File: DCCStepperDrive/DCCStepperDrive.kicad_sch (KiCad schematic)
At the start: 34 parts, among them J1 12v, J2 CBUS, J3 5V select, J4 DCC, J5 Grove 2mm, J6 GROVE-CONNECTOR-DIP_4P-2.0_, J7 Sensor, J8 Motor, J9 Mode Select, Q1 DMG2305UX-7, SW1 SW_Push, U1 AMS1117-3.3, U2 AMS1117-5.0, U3 6N137, U4 Pico

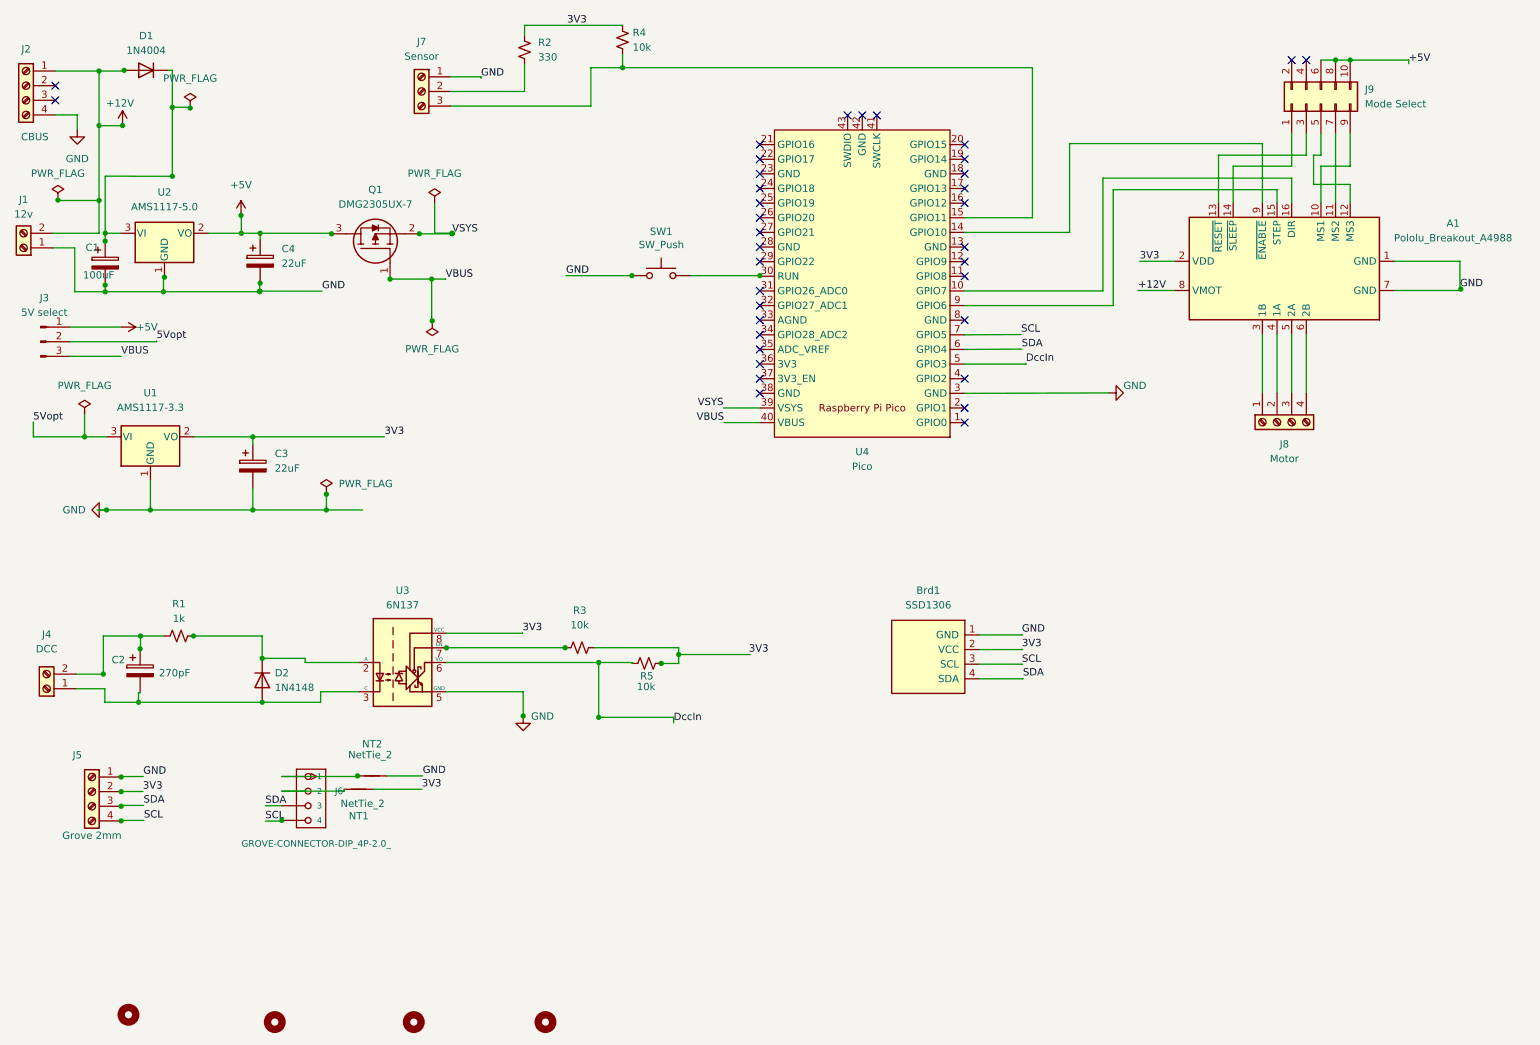
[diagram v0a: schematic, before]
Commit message: 19:27 Arrakis.local
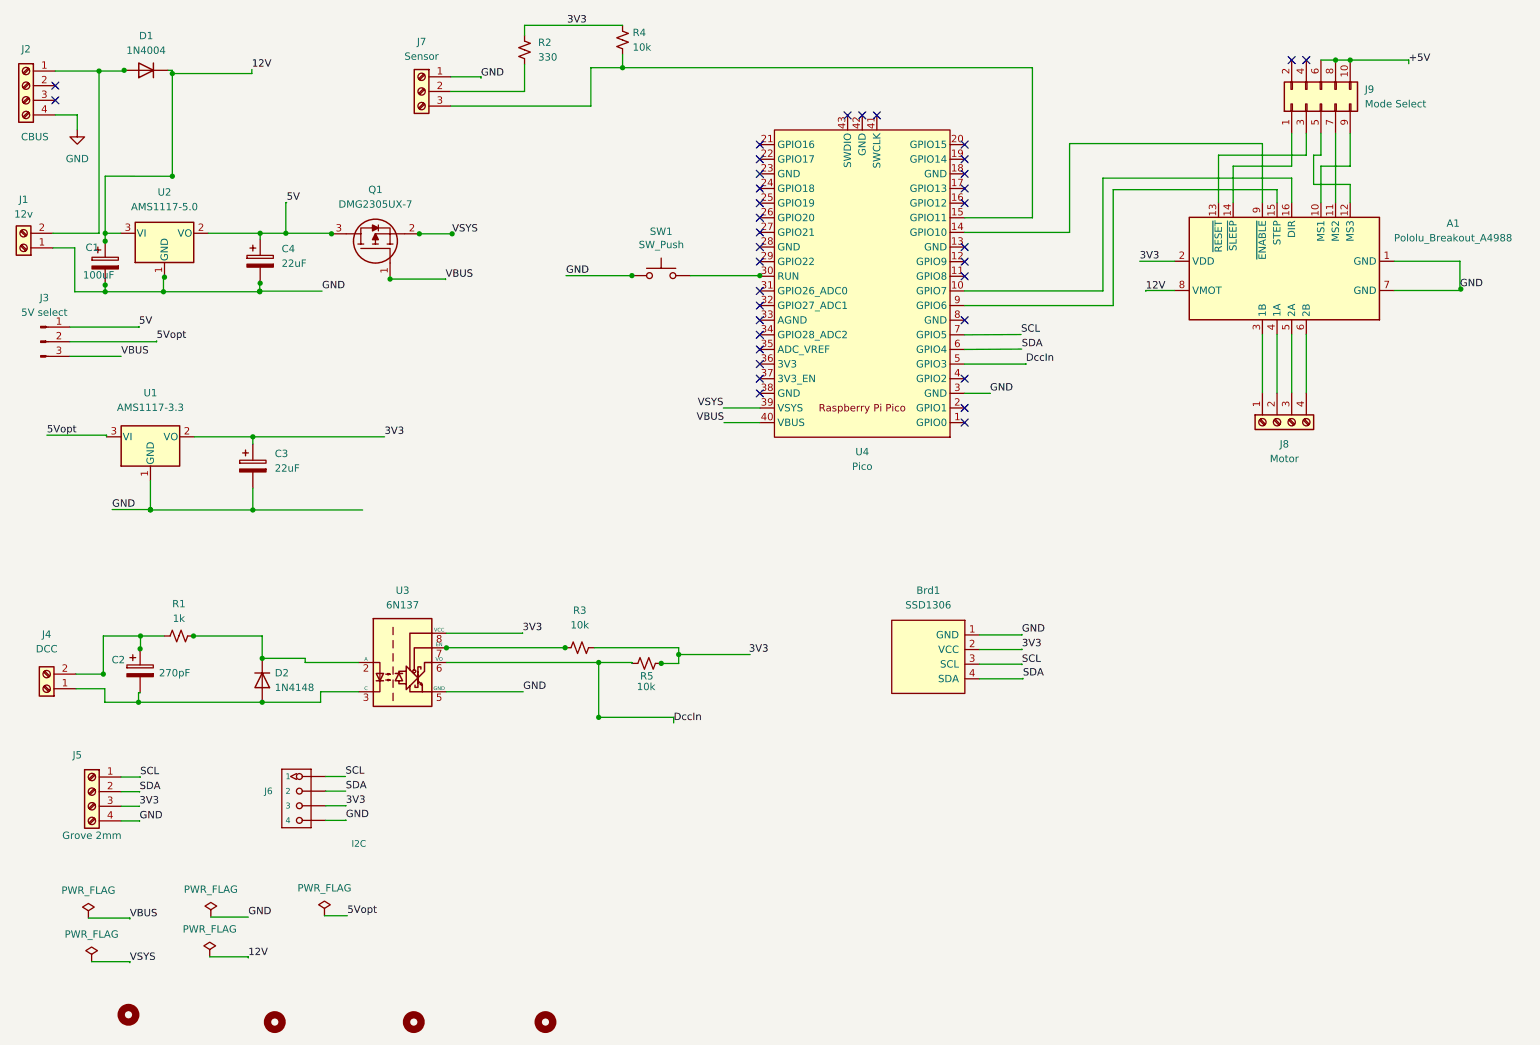
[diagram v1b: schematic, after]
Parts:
- removed NT1, NT2: NetTie_2, NetTie:NetTie-2_SMD_Pad0.5mm, symbol Device:NetTie_2
- J6: value GROVE-CONNECTOR-DIP_4P-2.0_ -> I2C
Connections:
- net +5V: no longer C4.1, J3.1 (Pin_1), Q1.3, U2.2 (VO)
- net 3V3: now also J5.3 (Pin_3), J6.3; no longer J5.2 (Pin_2)
- net GND: now also J5.4 (Pin_4), J6.4; no longer J5.1 (Pin_1)
- net SCL: now also J5.1 (Pin_1), J6.1; no longer J5.4 (Pin_4), J6.4
- net SDA: now also J5.2 (Pin_2), J6.2; no longer J5.3 (Pin_3), J6.3
- net 12V: now reaches C1.1, D1.1 (K), U2.3 (VI)
- net 12V: now also A1.8 (VMOT)
- net +12V: no longer names the net of D1.2 (A), J1.2 (Pin_2), J2.1 (Pin_1)
- net +12V: no longer A1.8 (VMOT)
- new net 5V: C4.1, J3.1 (Pin_1), Q1.3, U2.2 (VO)
